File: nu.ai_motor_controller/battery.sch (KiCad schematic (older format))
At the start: 36 parts

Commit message: automated commit
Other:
- note added: "Replace PTHs with connector symbol"
- note removed: "Decide whether to use cable assemblies or through hole xt60 connectors"
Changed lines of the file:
@@
 $EndComp
 Text Notes 975  2400 0    50   ~ 0
-Decide whether to use cable assemblies or through hole xt60 connectors
+Replace PTHs with connector symbol
 $Comp
 L custom:RA_SLIDE_SWITCH_DPDT SW?

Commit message: automated commit
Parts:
- removed J? (x4): PTH_3_mm, symbol custom:PTH_3_mm
- added J? (x2): XT60_RA_MALE, custom:XT60PW, symbol custom:XT60_RA_MALE
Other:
- note removed: "Replace PTHs with connector symbol"
- note removed: "XT60 MALE CABLE ASSEMBLY.\nADD 4 mm STRAIN RELIEF HOLES.\nINDICATE POS AND NEG\nON SILKSCREEN"
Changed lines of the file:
@@
 	1    0    0    -1
-$EndComp
-$Comp
-L custom:PTH_3_mm J?
-U 1 1 5C5B0327
-P 1575 3725
-AR Path="/5C5B0327" Ref="J?"  Part="1"
-AR Path="/5C100B31/5C5B0327" Ref="J?"  Part="1"
-AR Path="/5C5AE643/5C5B0327" Ref="J?"  Part="1"
-F 0 "J?" H 1725 3725 50  0000 C CNN
-F 1 "PTH_3_mm" H 1575 3625 50  0000 C CNN
-F 2 "" H 1575 3725 50  0001 C CNN
-F 3 "" H 1575 3725 50  0001 C CNN
-	1    1575 3725
-	-1   0    0    -1
-$EndComp
-$Comp
-L custom:PTH_3_mm J?
-U 1 1 5C5B032E
-P 1575 3475
-AR Path="/5C5B032E" Ref="J?"  Part="1"
-AR Path="/5C100B31/5C5B032E" Ref="J?"  Part="1"
-AR Path="/5C5AE643/5C5B032E" Ref="J?"  Part="1"
-F 0 "J?" H 1725 3475 50  0000 C CNN
-F 1 "PTH_3_mm" H 1575 3375 50  0000 C CNN
-F 2 "" H 1575 3475 50  0001 C CNN
-F 3 "" H 1575 3475 50  0001 C CNN
-	1    1575 3475
-	-1   0    0    -1
 $EndComp
 Text Notes 1750 1550 0    67   ~ 0
 INDICATE POS AND NEG\nON SILKSCREEN
-Text Notes 1050 4575 0    67   ~ 0
-XT60 MALE CABLE ASSEMBLY.\nADD 4 mm STRAIN RELIEF HOLES.\nINDICATE POS AND NEG\nON SILKSCREEN
+Text Notes 1175 4150 0    67   ~ 0
+INDICATE POS AND NEG\nON SILKSCREEN
 Wire Wire Line
 	1625 1225 1575 1225
@@
 L power:GND #PWR?
 U 1 1 5C5B046C
-P 1925 3850
-F 0 "#PWR?" H 1925 3600 50  0001 C CNN
-F 1 "GND" H 1925 3700 50  0000 C CNN
-F 2 "" H 1925 3850 50  0001 C CNN
-F 3 "" H 1925 3850 50  0001 C CNN
-	1    1925 3850
-	1    0    0    -1
-$EndComp
-Wire Wire Line
-	1925 3850 1925 3725
-Wire Wire Line
-	1725 3725 1925 3725
+P 1925 3700
+F 0 "#PWR?" H 1925 3450 50  0001 C CNN
+F 1 "GND" H 1925 3550 50  0000 C CNN
+F 2 "" H 1925 3700 50  0001 C CNN
+F 3 "" H 1925 3700 50  0001 C CNN
+	1    1925 3700
+	1    0    0    -1
+$EndComp
+Wire Wire Line
+	1925 3700 1925 3575
+Wire Wire Line
+	1725 3575 1925 3575
 $Comp
 L power:GND #PWR?
@@
 Wire Wire Line
 	1350 1125 1350 1025
-$Comp
-L custom:PTH_3_mm J?
-U 1 1 5C5B04AD
-P 1575 2775
-AR Path="/5C5B04AD" Ref="J?"  Part="1"
-AR Path="/5C100B31/5C5B04AD" Ref="J?"  Part="1"
-AR Path="/5C5AE643/5C5B04AD" Ref="J?"  Part="1"
-F 0 "J?" H 1725 2775 50  0000 C CNN
-F 1 "PTH_3_mm" H 1575 2675 50  0000 C CNN
-F 2 "" H 1575 2775 50  0001 C CNN
-F 3 "" H 1575 2775 50  0001 C CNN
-	1    1575 2775
-	-1   0    0    -1
-$EndComp
-$Comp
-L custom:PTH_3_mm J?
-U 1 1 5C5B04B4
-P 1575 2525
-AR Path="/5C5B04B4" Ref="J?"  Part="1"
-AR Path="/5C100B31/5C5B04B4" Ref="J?"  Part="1"
-AR Path="/5C5AE643/5C5B04B4" Ref="J?"  Part="1"
-F 0 "J?" H 1725 2525 50  0000 C CNN
-F 1 "PTH_3_mm" H 1575 2425 50  0000 C CNN
-F 2 "" H 1575 2525 50  0001 C CNN
-F 3 "" H 1575 2525 50  0001 C CNN
-	1    1575 2525
-	-1   0    0    -1
-$EndComp
-Wire Wire Line
-	1725 2525 2100 2525
-Wire Wire Line
-	1725 2775 1925 2775
-Wire Wire Line
-	1925 2775 1925 3725
-Connection ~ 1925 3725
-Wire Wire Line
-	2100 2525 2100 3475
+Wire Wire Line
+	1725 2950 2100 2950
+Wire Wire Line
+	1725 3050 1925 3050
+Wire Wire Line
+	1925 3050 1925 3575
+Connection ~ 1925 3575
+Wire Wire Line
+	2100 2950 2100 3475
 Connection ~ 2100 3475
 Wire Wire Line
@@
 	0    1    -1   0
 $EndComp
-Text Notes 975  2400 0    50   ~ 0
-Replace PTHs with connector symbol
 $Comp
 L custom:RA_SLIDE_SWITCH_DPDT SW?
@@
 NoConn ~ 3175 3575
 NoConn ~ 3175 3175
+$Comp
+L custom:XT60_RA_MALE J?
+U 1 1 5C521AAF
+P 1625 2950
+F 0 "J?" H 1575 3050 50  0000 L BNN
+F 1 "XT60_RA_MALE" H 1425 2550 50  0001 L BNN
+F 2 "custom:XT60PW" H 1425 2650 50  0001 L BNN
+F 3 "/home/dj/datasheets/XT60PW.pdf" H 1425 2450 50  0001 L BNN
+F 4 "XT60" H 1525 2750 50  0000 L BNN "Text"
+	1    1625 2950
+	1    0    0    -1
+$EndComp
+$Comp
+L custom:XT60_RA_MALE J?
+U 1 1 5C521B98
+P 1625 3475
+F 0 "J?" H 1575 3575 50  0000 L BNN
+F 1 "XT60_RA_MALE" H 1425 3075 50  0001 L BNN
+F 2 "custom:XT60PW" H 1425 3175 50  0001 L BNN
+F 3 "/home/dj/datasheets/XT60PW.pdf" H 1425 2975 50  0001 L BNN
+F 4 "XT60" H 1525 3275 50  0000 L BNN "Text"
+	1    1625 3475
+	1    0    0    -1
+$EndComp
 $EndSCHEMATC

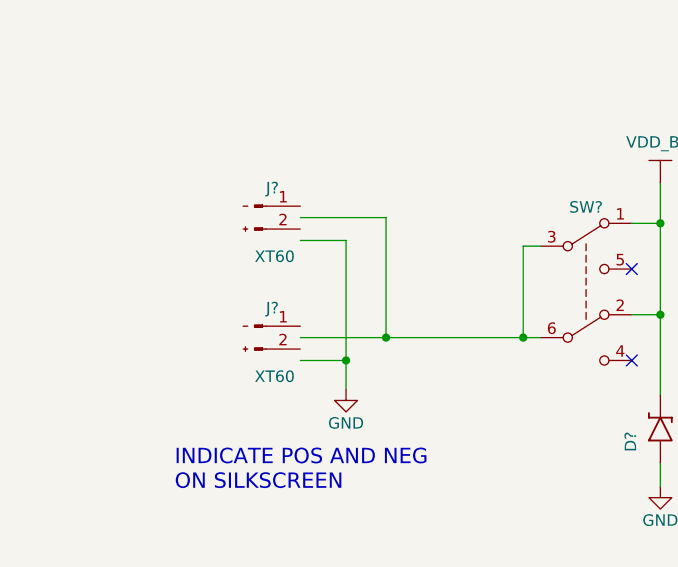
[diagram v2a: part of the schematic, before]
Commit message: automated commit
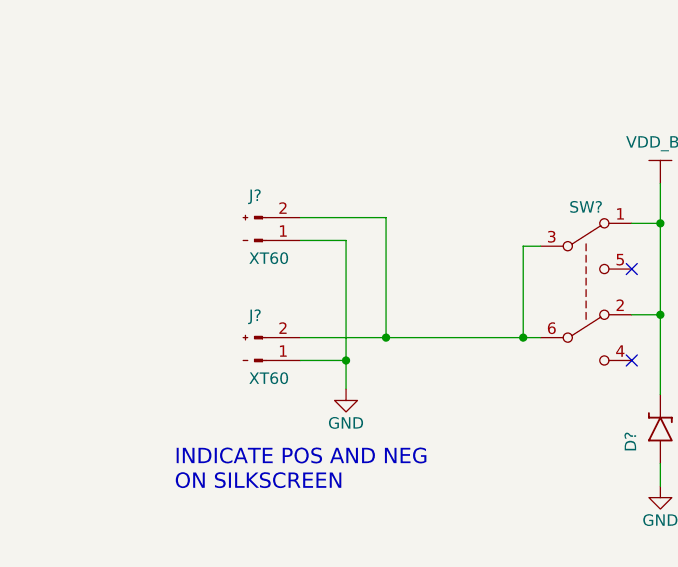
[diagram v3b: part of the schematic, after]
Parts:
- removed J?: XT60_RA_MALE, custom:XT60PW, symbol custom:XT60_RA_MALE
- added J?: XT60_RA_MALE, custom:XT60PW, symbol custom:XT60_RA_MALE
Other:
- moved on the sheet: J?
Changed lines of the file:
@@
 L custom:XT60_RA_MALE J?
 U 1 1 5C521AAF
-P 1625 2950
-F 0 "J?" H 1575 3050 50  0000 L BNN
-F 1 "XT60_RA_MALE" H 1425 2550 50  0001 L BNN
-F 2 "custom:XT60PW" H 1425 2650 50  0001 L BNN
-F 3 "/home/dj/datasheets/XT60PW.pdf" H 1425 2450 50  0001 L BNN
-F 4 "XT60" H 1525 2750 50  0000 L BNN "Text"
-	1    1625 2950
-	1    0    0    -1
+P 1625 3000
+F 0 "J?" H 1500 2825 50  0000 L BNN
+F 1 "XT60_RA_MALE" H 1425 2600 50  0001 L BNN
+F 2 "custom:XT60PW" H 1425 2700 50  0001 L BNN
+F 3 "/home/dj/datasheets/XT60PW.pdf" H 1425 2500 50  0001 L BNN
+F 4 "XT60" H 1500 3100 50  0000 L BNN "Text"
+	1    1625 3000
+	1    0    0    1
 $EndComp
 $Comp
 L custom:XT60_RA_MALE J?
-U 1 1 5C521B98
-P 1625 3475
-F 0 "J?" H 1575 3575 50  0000 L BNN
-F 1 "XT60_RA_MALE" H 1425 3075 50  0001 L BNN
-F 2 "custom:XT60PW" H 1425 3175 50  0001 L BNN
-F 3 "/home/dj/datasheets/XT60PW.pdf" H 1425 2975 50  0001 L BNN
-F 4 "XT60" H 1525 3275 50  0000 L BNN "Text"
-	1    1625 3475
-	1    0    0    -1
+U 1 1 5C54FBBA
+P 1625 3525
+F 0 "J?" H 1500 3350 50  0000 L BNN
+F 1 "XT60_RA_MALE" H 1425 3125 50  0001 L BNN
+F 2 "custom:XT60PW" H 1425 3225 50  0001 L BNN
+F 3 "/home/dj/datasheets/XT60PW.pdf" H 1425 3025 50  0001 L BNN
+F 4 "XT60" H 1500 3625 50  0000 L BNN "Text"
+	1    1625 3525
+	1    0    0    1
 $EndComp
 $EndSCHEMATC
